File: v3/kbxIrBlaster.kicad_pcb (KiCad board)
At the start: 2 copper layers, 84.3 x 33 mm, 47 parts, among them J1 CH1, J2 CH2, J3 CH3, J4 CH4, J5 Conn_01x06, J6 Conn_01x15, J7 Conn_01x15, J8 Barrel_Jack_Switch, J9 USB_B_Micro, Q1 2N7002, Q2 2N7002, Q3 2N7002, Q4 2N7002, SW1 RESET, SW2 BOOT, U1 TSOP382xx, U2 TSOP382xx, U3 ESP32-WROOM-32D, U4 AP2112K-3.3

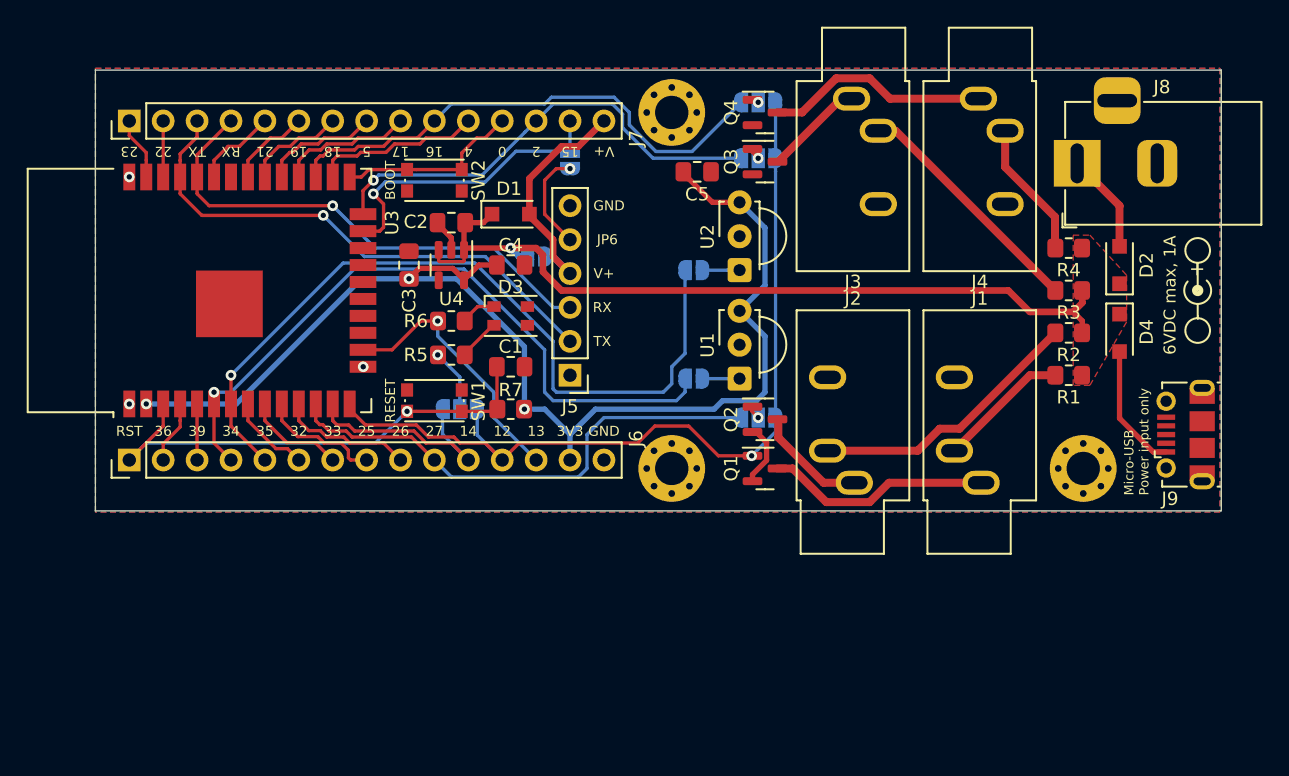
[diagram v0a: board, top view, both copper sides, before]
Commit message: Update with v3
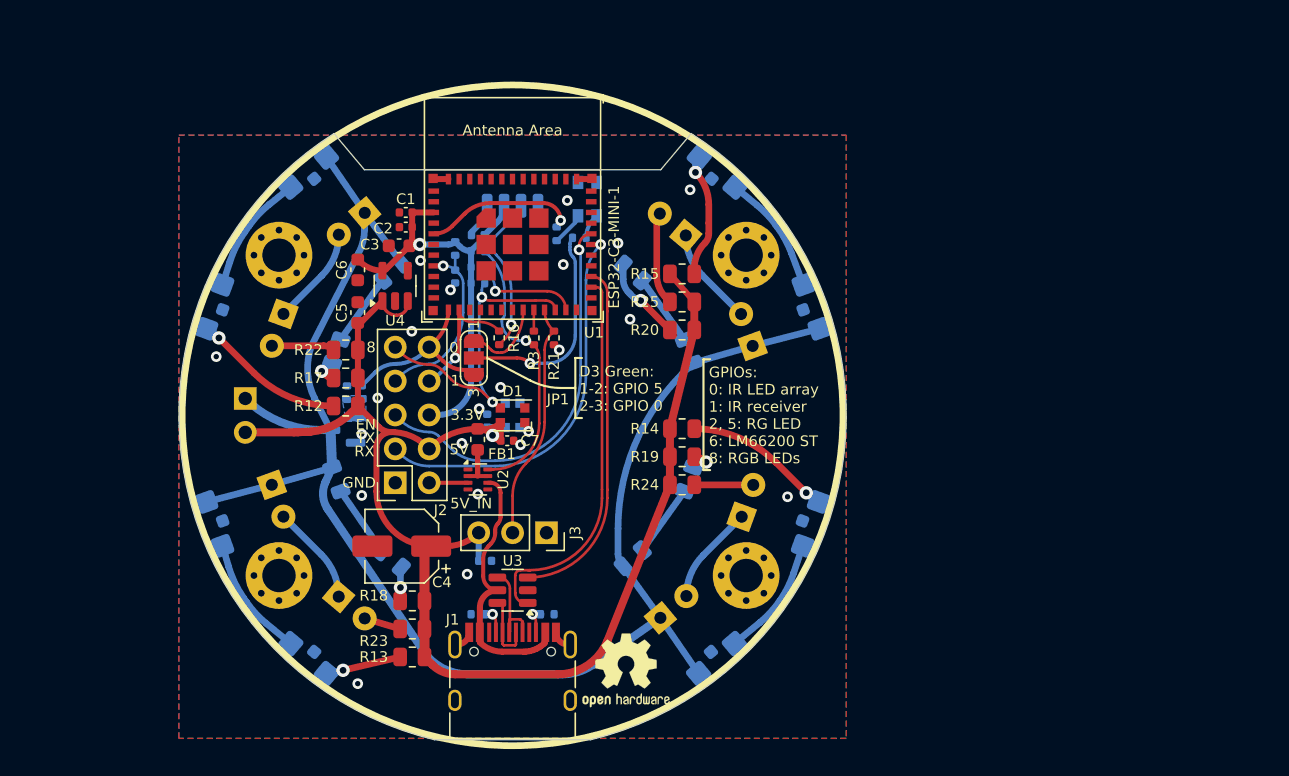
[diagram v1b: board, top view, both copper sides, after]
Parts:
- removed J5: Conn_01x06, Connector_PinHeader_2.54mm:PinHeader_1x06_P2.54mm_Vertical
- removed J6, J7: Conn_01x15, Connector_PinHeader_2.54mm:PinHeader_1x15_P2.54mm_Vertical
- removed J8: Barrel_Jack_Switch, Connector_BarrelJack:BarrelJack_Horizontal
- removed J9: USB_B_Micro, Connector_USB:USB_Micro-B_Molex-105017-0001
- removed JP2, JP3, JP8: SolderJumper_3_Open, Jumper:SolderJumper-3_P1.3mm_Open_RoundedPad1.0x1.5mm
- removed JP4, JP5, JP6, JP7: SolderJumper_2_Open, Jumper:SolderJumper-2_P1.3mm_Open_RoundedPad1.0x1.5mm
- removed Q2, Q3, Q4: 2N7002, Package_TO_SOT_SMD:SOT-23
- removed the REF** at (201.2, 80.6)
- removed SW1: RESET, Button_Switch_SMD:SW_Push_1P1T_NO_CK_KMR2
- removed SW2: BOOT, Button_Switch_SMD:SW_Push_1P1T_NO_CK_KMR2
- added C10: 100n, Capacitor_SMD:C_0402_1005Metric, B.Cu at (147.4, 76.5)
- added C11: 1u, Capacitor_SMD:C_0402_1005Metric, B.Cu at (147.9, 100.9)
- added C6: 10u/20%, Capacitor_SMD:C_0603_1608Metric, F.Cu at (138.4, 79.1)
- added C7: 100n, Capacitor_SMD:C_0402_1005Metric, F.Cu at (149.6, 91.9)
- added C8: 1u, Capacitor_SMD:C_0402_1005Metric, B.Cu at (145.7, 79.6)
- added C9: 100n, Capacitor_SMD:C_0402_1005Metric, B.Cu at (148.1, 90.4)
- added D10: VSMB10940, LED_SMD:LED_Kingbright_KPA-3010_3x2x1mm, B.Cu at (165.7, 71.4)
- added D11: VSMB10940, LED_SMD:LED_Kingbright_KPA-3010_3x2x1mm, B.Cu at (172.8, 81.7)
- added D12: APT2012F3C, LED_SMD:LED_0805_2012Metric, B.Cu at (136.8, 85.2)
- added D13: APT2012F3C, LED_SMD:LED_0805_2012Metric, B.Cu at (141.0, 79.2)
- added D14: APT2012F3C, LED_SMD:LED_0805_2012Metric, B.Cu at (140.9, 100.8)
- added D15: APT2012F3C, LED_SMD:LED_0805_2012Metric, B.Cu at (136.8, 94.8)
- added D16: APT2012F3C, LED_SMD:LED_0805_2012Metric, B.Cu at (163.2, 94.8)
- added D17: APT2012F3C, LED_SMD:LED_0805_2012Metric, B.Cu at (159.0, 100.7)
- added D18: APT2012F3C, LED_SMD:LED_0805_2012Metric, B.Cu at (159.0, 79.3)
- added D19: APT2012F3C, LED_SMD:LED_0805_2012Metric, B.Cu at (163.2, 85.2)
- added D20: CH1, LED_THT:LED_D5.0mm, B.Cu at (132.8, 82.4)
- added D21: CH1, LED_THT:LED_D5.0mm, B.Cu at (138.9, 74.8)
- added D22: CH1, LED_THT:LED_D5.0mm, B.Cu at (137.0, 103.6)
- added D23: CH1, LED_THT:LED_D5.0mm, B.Cu at (132.0, 95.2)
- added D24: CH1, LED_THT:LED_D5.0mm, B.Cu at (167.2, 97.6)
- added D25: CH1, LED_THT:LED_D5.0mm, B.Cu at (161.1, 105.2)
- added D26: CH1, LED_THT:LED_D5.0mm, B.Cu at (163.0, 76.5)
- added D27: CH1, LED_THT:LED_D5.0mm, B.Cu at (168.0, 84.8)
- added D5: VSMB10940, LED_SMD:LED_Kingbright_KPA-3010_3x2x1mm, B.Cu at (134.4, 71.4)
- added D6: VSMB10940, LED_SMD:LED_Kingbright_KPA-3010_3x2x1mm, B.Cu at (134.4, 108.6)
- added D7: VSMB10940, LED_SMD:LED_Kingbright_KPA-3010_3x2x1mm, B.Cu at (127.2, 98.3)
- added D8: VSMB10940, LED_SMD:LED_Kingbright_KPA-3010_3x2x1mm, B.Cu at (172.8, 98.3)
- added D9: VSMB10940, LED_SMD:LED_Kingbright_KPA-3010_3x2x1mm, B.Cu at (165.6, 108.6)
- added FB1: 600R/1A, Inductor_SMD:L_0603_1608Metric, F.Cu at (147.4, 91.8)
- added H4: MountingHole_Pad, MountingHole:MountingHole_2.5mm_Pad_Via, F.Cu at (167.5, 102.0)
- added R10: 100R, Resistor_SMD:R_0402_1005Metric, B.Cu at (138.7, 88.3)
- added R11: 10k, Resistor_SMD:R_0402_1005Metric, B.Cu at (137.6, 88.3)
- added R12: 47, Resistor_SMD:R_0805_2012Metric, F.Cu at (137.5, 89.3)
- added R13: 47, Resistor_SMD:R_0805_2012Metric, F.Cu at (142.5, 108.1)
- added R14: 47, Resistor_SMD:R_0805_2012Metric, F.Cu at (162.7, 91.0)
- added R15: 47, Resistor_SMD:R_0805_2012Metric, F.Cu at (162.7, 79.4)
- added R16: 100R, Resistor_SMD:R_0402_1005Metric, F.Cu at (149.0, 84.2)
- added R17: 56, Resistor_SMD:R_0805_2012Metric, F.Cu at (137.5, 87.2)
- added R18: 56, Resistor_SMD:R_0805_2012Metric, F.Cu at (142.5, 103.9)
- added R19: 56, Resistor_SMD:R_0805_2012Metric, F.Cu at (162.7, 93.1)
- added R20: 56, Resistor_SMD:R_0805_2012Metric, F.Cu at (162.7, 83.6)
- added R21: 10k, Resistor_SMD:R_0402_1005Metric, F.Cu at (153.1, 84.2)
- added R22: 27, Resistor_SMD:R_0805_2012Metric, F.Cu at (137.5, 85.1)
- added R23: 27, Resistor_SMD:R_0805_2012Metric, F.Cu at (142.5, 106.0)
- added R24: 27, Resistor_SMD:R_0805_2012Metric, F.Cu at (162.7, 95.2)
- added R25: 27, Resistor_SMD:R_0805_2012Metric, F.Cu at (162.7, 81.5)
- added R8: 100R, Resistor_SMD:R_0402_1005Metric, B.Cu at (155.0, 76.7)
- added R9: 100R, Resistor_SMD:R_0402_1005Metric, B.Cu at (153.3, 76.4)
- added REF**: OSHW-Logo2_7.3x6mm_SilkScreen, Symbol:OSHW-Logo2_7.3x6mm_SilkScreen, F.Cu at (158.5, 109.1)
- added REF**: OSHW-Logo2_7.3x6mm_SilkScreen, Symbol:OSHW-Logo2_7.3x6mm_SilkScreen, B.Cu at (150.0, 111.4)
- added U5: TSOP752xx, kbxIrBlaster:Vishay_TSOP752_Horizontal, B.Cu at (150.0, 73.5)
- C1: value 1 uF -> 100n; footprint Capacitor_SMD:C_0805_2012Metric_Pad1.18x1.45mm_HandSolder -> Capacitor_SMD:C_0402_1005Metric
- C2: value 10 uF -> 1u; footprint Capacitor_SMD:C_0805_2012Metric_Pad1.18x1.45mm_HandSolder -> Capacitor_SMD:C_0402_1005Metric
- C3, C5: value 10 uF -> 10u/20%; footprint Capacitor_SMD:C_0805_2012Metric_Pad1.18x1.45mm_HandSolder -> Capacitor_SMD:C_0603_1608Metric
- C4: value 10 uF -> 100u; footprint Capacitor_SMD:C_0805_2012Metric_Pad1.18x1.45mm_HandSolder -> Capacitor_SMD:CP_Elec_5x5.4
- D1: value MBR120 -> WS2812B; footprint Diode_SMD:D_SOD-123F -> LED_SMD:LED_WS2812B-2020_PLCC4_2.0x2.0mm
- D2: value MBR120 -> WS2812B; footprint Diode_SMD:D_SOD-123F -> LED_SMD:LED_WS2812B-2020_PLCC4_2.0x2.0mm; moved to B.Cu
- D3: value LED_Dual_AACC -> HW_LED; moved to B.Cu
- D4: value MBR120 -> VSMB10940; footprint Diode_SMD:D_SOD-123F -> LED_SMD:LED_Kingbright_KPA-3010_3x2x1mm; moved to B.Cu
- J1: value CH1 -> HRO TYPE-C 31-M-12; footprint Connector_Audio:Jack_3.5mm_CUI_SJ1-3533NG_Horizontal -> Connector_USB:USB_C_Receptacle_HRO_TYPE-C-31-M-12
- J2: value CH2 -> POWER_IO; footprint Connector_Audio:Jack_3.5mm_CUI_SJ1-3533NG_Horizontal -> Connector_PinSocket_2.54mm:PinSocket_2x05_P2.54mm_Vertical
- J3: value CH3 -> RF; footprint Connector_Audio:Jack_3.5mm_CUI_SJ1-3533NG_Horizontal -> Connector_PinSocket_2.54mm:PinSocket_1x03_P2.54mm_Vertical
- J4: value CH4 -> EXT_LED; footprint Connector_Audio:Jack_3.5mm_CUI_SJ1-3533NG_Horizontal -> Connector_PinSocket_2.54mm:PinSocket_1x02_P2.54mm_Vertical; moved to B.Cu
- JP1: value SolderJumper_3_Open -> LED_SEL; footprint Jumper:SolderJumper-3_P1.3mm_Open_RoundedPad1.0x1.5mm -> Jumper:SolderJumper-3_P1.3mm_Open_RoundedPad1.0x1.5mm_NumberLabels; moved to F.Cu
- Q1: value 2N7002 -> PMV164ENEAR; moved to B.Cu
- R1, R2: value 27 -> 5k1; footprint Resistor_SMD:R_0805_2012Metric_Pad1.20x1.40mm_HandSolder -> Resistor_SMD:R_0402_1005Metric; moved to B.Cu
- R3: value 27 -> 100R; footprint Resistor_SMD:R_0805_2012Metric_Pad1.20x1.40mm_HandSolder -> Resistor_SMD:R_0402_1005Metric
- R4: value 27 -> 10k; footprint Resistor_SMD:R_0805_2012Metric_Pad1.20x1.40mm_HandSolder -> Resistor_SMD:R_0402_1005Metric; moved to B.Cu
- R5, R6: value 1K -> 10k; footprint Resistor_SMD:R_0805_2012Metric_Pad1.20x1.40mm_HandSolder -> Resistor_SMD:R_0402_1005Metric; moved to B.Cu
- R7: value 10K -> 10k; footprint Resistor_SMD:R_0805_2012Metric_Pad1.20x1.40mm_HandSolder -> Resistor_SMD:R_0402_1005Metric; moved to B.Cu
- U1: value TSOP382xx -> ESP32-C3-MINI-1; footprint OptoDevice:Vishay_MINICAST-3Pin -> PCM_Espressif:ESP32-C3-MINI-1
- U2: value TSOP382xx -> LM66200; footprint OptoDevice:Vishay_MINICAST-3Pin -> Package_TO_SOT_SMD:SOT-583-8
- U3: value ESP32-WROOM-32D -> USBLC6-2SC6; footprint RF_Module:ESP32-WROOM-32 -> Package_TO_SOT_SMD:SOT-23-6
- moved D4 68.3 mm to (127.2, 81.7), turned to -110 degrees
- moved H3 60.8 mm to (132.5, 102.0)
- moved J4 59.3 mm to (130.0, 88.7), turned to 180 degrees
- moved R2 49.0 mm to (147.4, 104.9)
- moved D2 46.8 mm to (150.0, 90.0), turned to -90 degrees
- moved R4 44.3 mm to (147.4, 77.7), turned to 0 degrees
- moved R1 43.0 mm to (152.6, 104.9), turned to 0 degrees
- moved R3 40.2 mm to (151.6, 84.2), turned to -90 degrees
- moved J3 39.7 mm to (152.5, 98.8), turned to -90 degrees
- moved J1 38.3 mm to (150.0, 110.3), turned to 0 degrees
- moved J2 34.4 mm to (141.2, 95.0)
- moved Q1 31.7 mm to (137.3, 91.1), turned to 180 degrees
- moved H1 31.3 mm to (132.5, 78.0)
- moved U3 30.4 mm to (150.0, 103.1), turned to 180 degrees
- moved C5 27.5 mm to (138.4, 82.3), turned to 90 degrees
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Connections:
- C1 pad 1: RESET -> +3.3V
- C2 pad 1: GND -> +3.3V
- C2 pad 2: +5V -> GND
- C3 pad 1: GND -> +3.3V
- C3 pad 2: +3V3 -> GND
- C4 pad 1: GND -> +5V
- C4 pad 2: +3V3 -> GND
- C5 pad 1: GND -> +5V
- C5 pad 2: +3V3 -> GND
- D1 pad 1: +5V -> Net-(D1-DOUT)
- D1 pad 2: +BATT -> GND
- D2 pad 1: +5V -> /LED_DOUT
- D2 pad 2: Net-(D2-Pad2) -> GND
- D3 pad 1: Net-(D3-Pad1) -> Net-(D3-A1)
- D3 pad 2: Net-(D3-Pad2) -> Net-(D3-A2)
- D4 pad 1: +5V -> Net-(D4-K)
- JP1 pad 1: GPIO27 -> /GPIO5
- JP1 pad 3: GPIO12 -> /GPIO0
- Q1 pad 1: GPIO12 -> /FET_GATE
- Q1 pad 3: FET1 -> /LED_K
- R1 pad 1: +5V -> /USB_CC2
- R1 pad 2: Net-(J1-PadT) -> GND
- R2 pad 1: +5V -> /USB_CC1
- R2 pad 2: Net-(J2-PadT) -> GND
- R3 pad 1: +5V -> /GPIO6
- R3 pad 2: Net-(J3-PadT) -> /ST
- R4 pad 1: +5V -> +3.3V
- R4 pad 2: Net-(J4-PadT) -> /ST
- R5 pad 1: Net-(JP8-Pad2) -> /ESP_EN
- R5 pad 2: Net-(D3-Pad2) -> +3.3V
- R6 pad 1: GPIO13 -> /GPIO9
- R6 pad 2: Net-(D3-Pad1) -> +3.3V
- R7 pad 1: +3V3 -> /GPIO8
- R7 pad 2: RESET -> +3.3V
- U1 pad 1: Net-(JP4-Pad1) -> GND
- U1 pad 3: +3V3 -> +3.3V
- U2 pad 1: Net-(JP5-Pad1) -> GND
- U2 pad 2: GND -> Net-(FB1-Pad1)
- U2 pad 3: +3V3 -> /PWR_EXT
- U3 pad 1: GND -> /ESP_USB_D-
- U3 pad 2: +3V3 -> GND
- U3 pad 3: RESET -> /ESP_USB_D+
- U3 pad 4: GPIO36 -> /USB_D+
- U3 pad 5: GPIO39 -> /USB_VBUS
- U3 pad 6: GPI34 -> /USB_D-
- U4 pad 5: +3V3 -> +3.3V
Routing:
- net /LED_K: track 0.00 -> 119.0 mm
- net +3V3: track 90.7 -> 0.00 mm, vias 3 -> 0
- net GPIO12: track 65.9 -> 0.00 mm, vias 1 -> 0
- net GPI35: track 59.2 -> 0.00 mm, vias 1 -> 0
- net GPI34: track 51.9 -> 0.00 mm, vias 1 -> 0
- net +5V: track 61.6 -> 111.1 mm
- net TXD: track 39.8 -> 0.00 mm, vias 1 -> 0
- net GPIO16: track 38.8 -> 0.00 mm
- net GPIO27: track 38.2 -> 0.00 mm
- net RXD: track 38.0 -> 0.00 mm, vias 1 -> 0
- net RESET: track 37.6 -> 0.00 mm, vias 1 -> 0
- net GPIO2: track 35.0 -> 0.00 mm, vias 1 -> 0
- net +3.3V: track 0.00 -> 32.5 mm, vias 0 -> 1
- net /ESP_U0_TXD: track 0.00 -> 29.5 mm, vias 0 -> 1
- net /ESP_U0_RXD: track 0.00 -> 29.1 mm, vias 0 -> 1
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- added copper zone on B.Cu, net /FET_GATE
- removed copper zone on F.Cu, net +5V
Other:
- board size 84.3 x 33 mm -> 50 x 45.4 mm
- board text added: "D3 Green: 1-2: GPIO 5 2-3: GPIO 0"
- board text added: "Designed by Keith Burzinski (@kbx81) in Chicago, Illinois v3 - December 2024"
- board text added: "GPIOs: 0: IR LED array 1: IR receiver 2, 5: RG LED 6: LM66200 ST 8: RGB LEDs"
- board text added: "Mini IR MegaBlaster with ESP32-C3"
- board text removed: "433 MHz Transmitter"
- board text removed: "Designed by Keith Burzinski (@kbx81) in Chicago, Illinois"
- board text removed: "ESP32 IR MegaBlaster and LED Controller v1.3"
- board text removed: "IR Receiver Disconnects: JP1 = U1 JP2 = U2 GPIO-to-LED Assignments: JP3 = D2, D6 JP4 = D3, D7 JP5 = D4, D8"
- board text removed: "Micro-USB Power input only"
